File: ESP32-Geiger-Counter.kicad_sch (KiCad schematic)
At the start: 0 parts

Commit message: save
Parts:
- added J1: USB_C_Receptacle_PowerOnly_6P, symbol Connector:USB_C_Receptacle_PowerOnly_6P
- added U1: TP4056-42-ESOP8, Package_SO:SOIC-8-1EP_3.9x4.9mm_P1.27mm_EP2.41x3.3mm_ThermalVias, symbol Battery_Management:TP4056-42-ESOP8
- added U2: ESP32-WROOM-32, RF_Module:ESP32-WROOM-32, symbol RF_Module:ESP32-WROOM-32
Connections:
- new net: U2.1 (GND), U2.15 (GND), U2.38 (GND), U2.39 (GND)
- new net: J1.A12 (GND), J1.B12 (GND)
- new net: J1.A9 (VBUS), J1.B9 (VBUS)
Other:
- title: (none) -> ESP32-based Geiger Counter

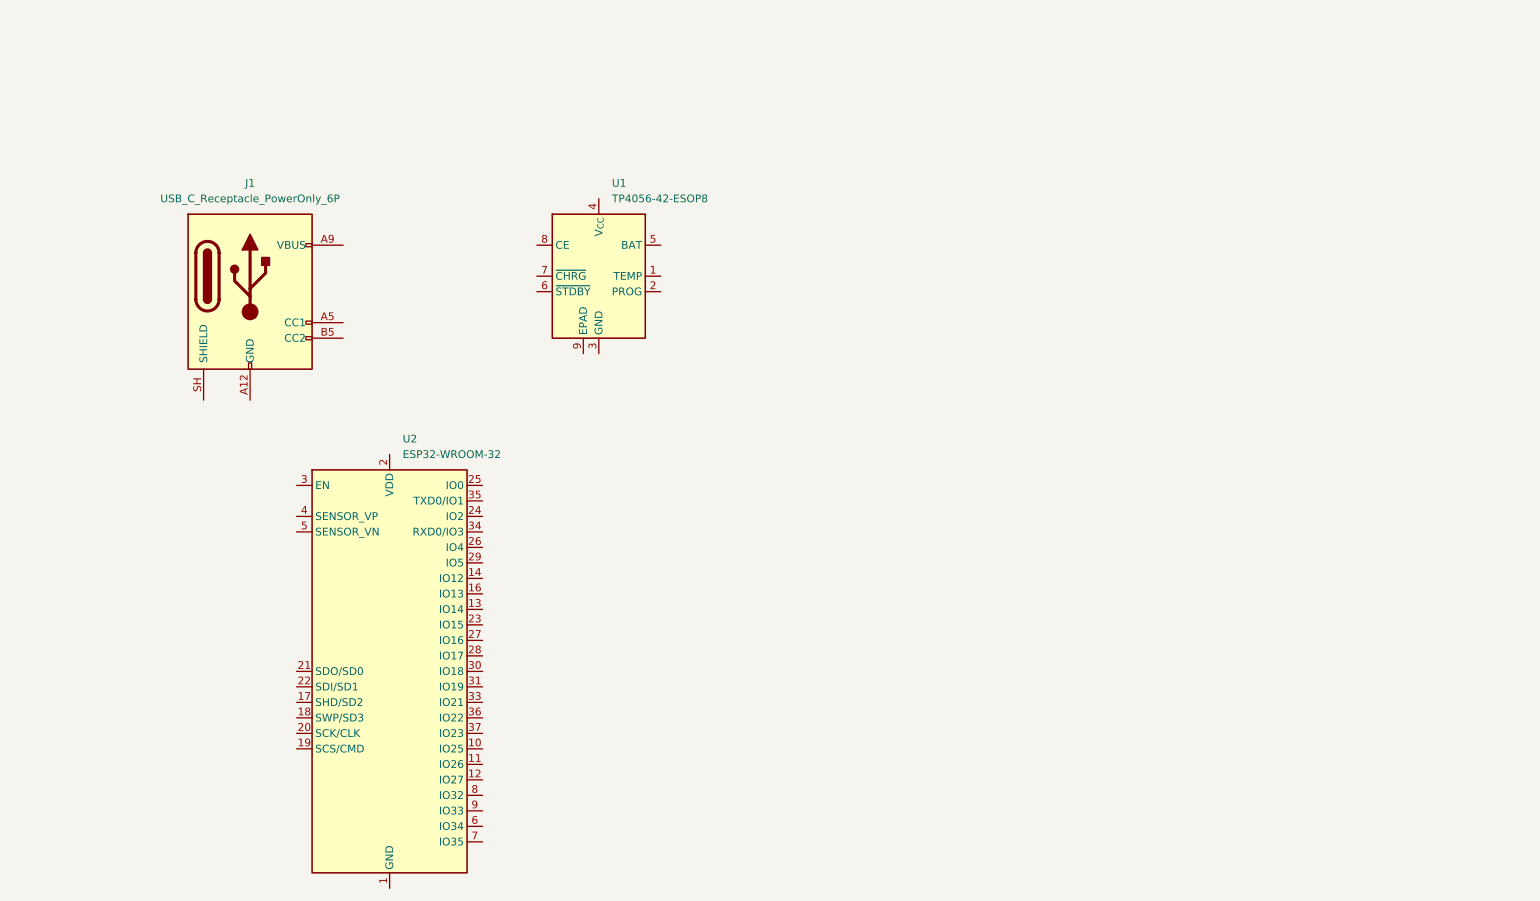
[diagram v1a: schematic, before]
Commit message: usb
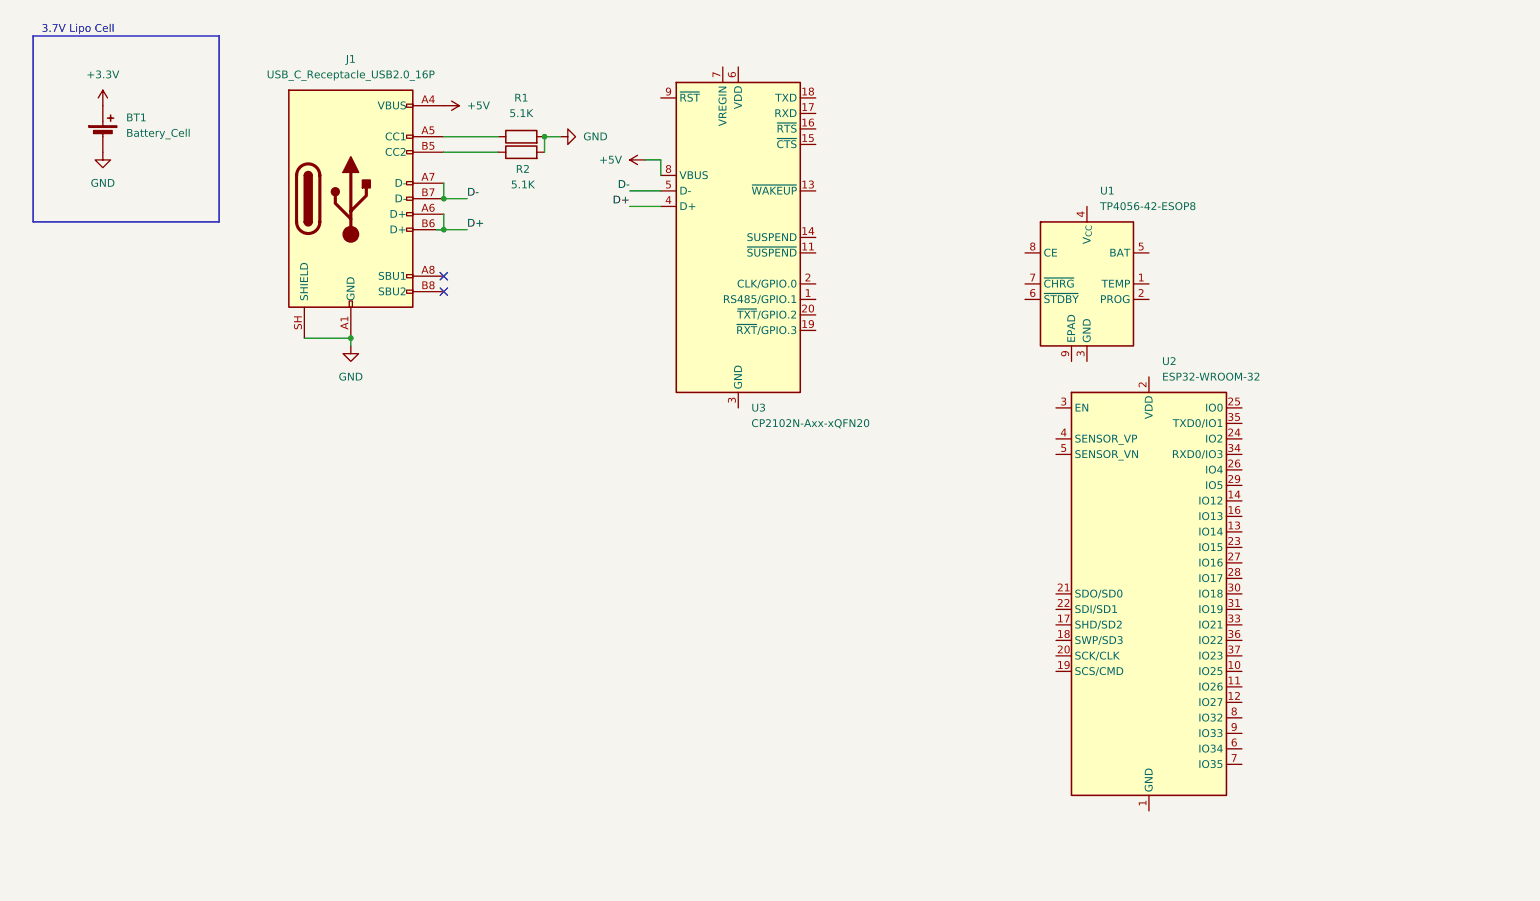
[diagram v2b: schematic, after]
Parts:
- removed J1: USB_C_Receptacle_PowerOnly_6P, symbol Connector:USB_C_Receptacle_PowerOnly_6P
- added BT1: Battery_Cell, Connector_JST:JST_PH_B2B-PH-K_1x02_P2.00mm_Vertical, symbol Device:Battery_Cell
- added J1: USB_C_Receptacle_USB2.0_16P, symbol Connector:USB_C_Receptacle_USB2.0_16P
- added R1, R2: 5.1K, symbol Device:R
- added U3: CP2102N-Axx-xQFN20, Package_DFN_QFN:SiliconLabs_QFN-20-1EP_3x3mm_P0.5mm, symbol Interface_USB:CP2102N-Axx-xQFN20
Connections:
- new net: J1.B5 (CC2), R2.1
- new net: J1.A5 (CC1), R1.1
- new net: U3.12 (GND), U3.21 (GND), U3.3 (GND)
- new net +3.3V: BT1.1 (+)
- new net +5V: J1.A4 (VBUS), J1.A9 (VBUS), J1.B4 (VBUS), J1.B9 (VBUS), U3.8 (VBUS)
- new net D+: J1.A6 (D+), J1.B6 (D+), U3.4 (D+)
- new net D-: J1.A7 (D-), J1.B7 (D-), U3.5 (D-)
- new net GND: BT1.2 (-), J1.A1 (GND), J1.A12 (GND), J1.B1 (GND), J1.B12 (GND), J1.SH (SHIELD), R1.2, R2.2
- no-connect marks 0 -> 2
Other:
- note added: "3.7V Lipo Cell"
- moved on the sheet: U1, U2

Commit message: saving
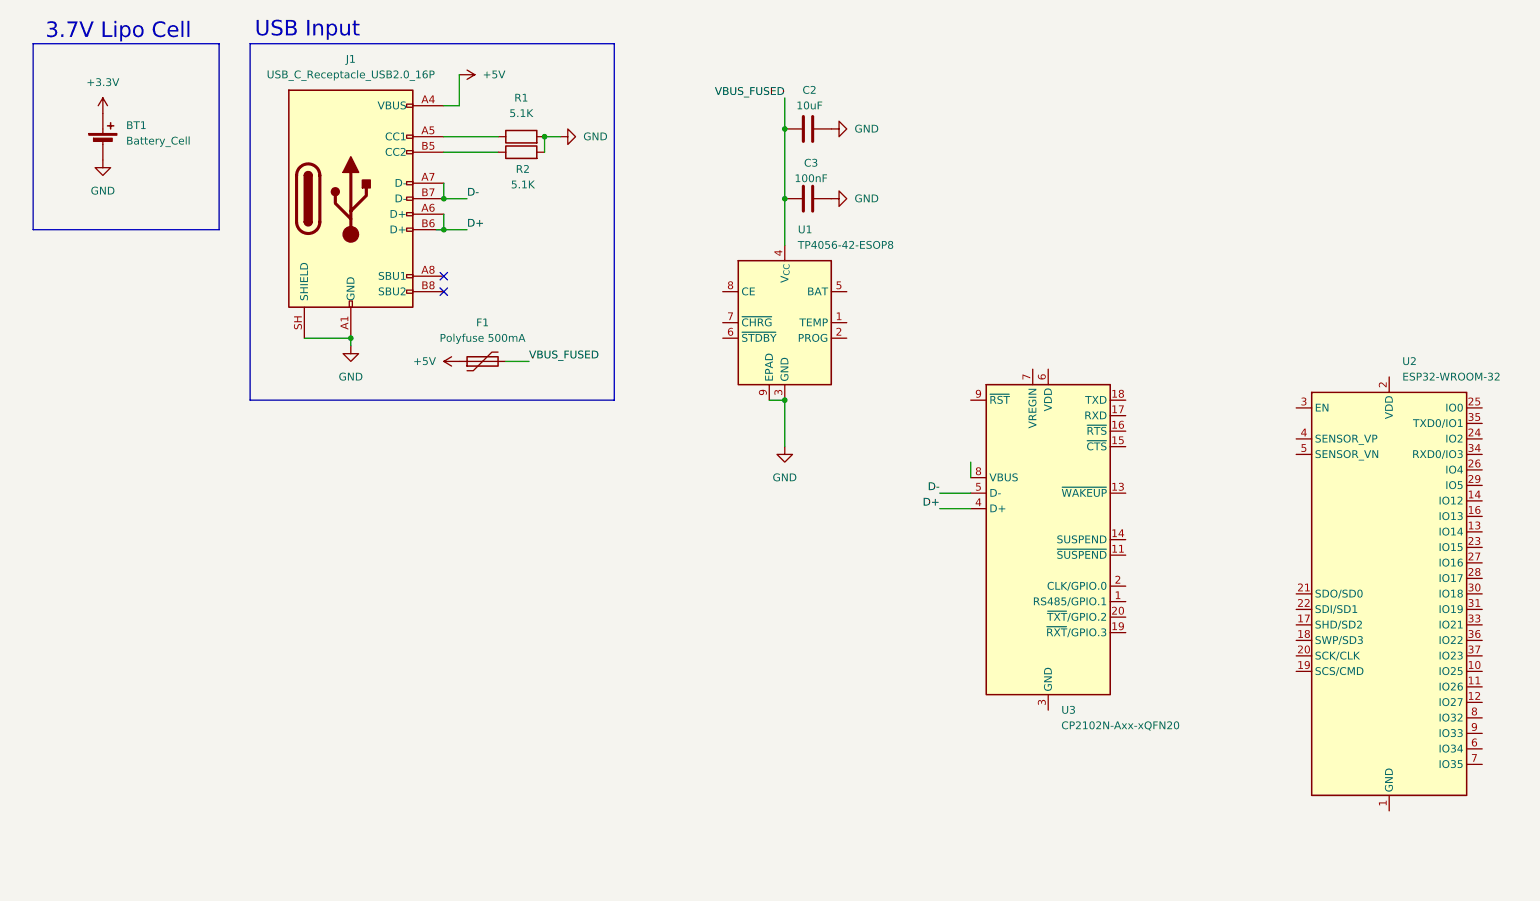
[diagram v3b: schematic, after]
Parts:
- added C2: 10uF, symbol Device:C
- added C3: 100nF, symbol Device:C
- added F1: Polyfuse 500mA, Fuse:Fuse_1812_4532Metric, symbol Device:Polyfuse
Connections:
- net +5V: now also F1.1; no longer U3.8 (VBUS)
- net GND: now also U1.3 (GND), U1.9 (EPAD), C2.2, C3.2
- net VBUS_FUSED: now reaches U1.4 (V_{CC})
- net VBUS_FUSED: now also C2.1, C3.1, F1.2
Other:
- note added: "USB Input"
- moved on the sheet: BT1, U1, U2, U3
